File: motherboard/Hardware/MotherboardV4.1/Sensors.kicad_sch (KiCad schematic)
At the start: 33 parts, among them J401 0, J5 0, J6 0, J7 0

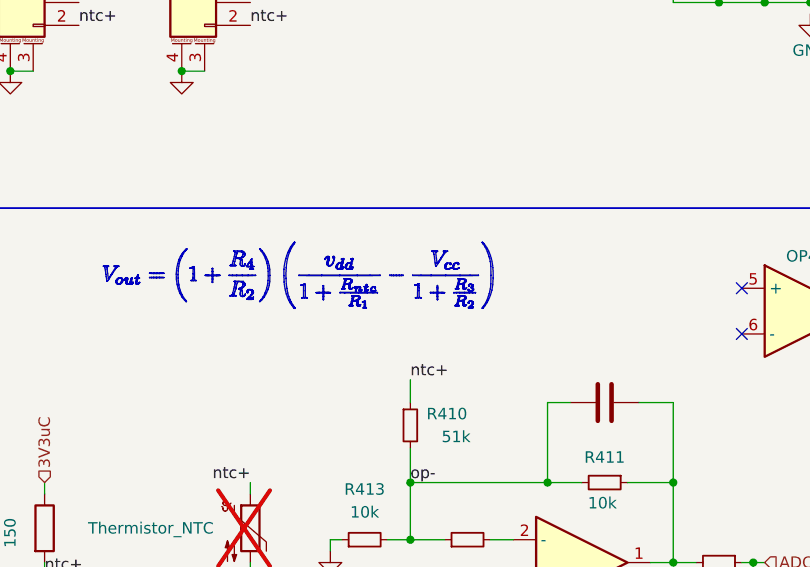
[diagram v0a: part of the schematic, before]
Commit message: working on thermal
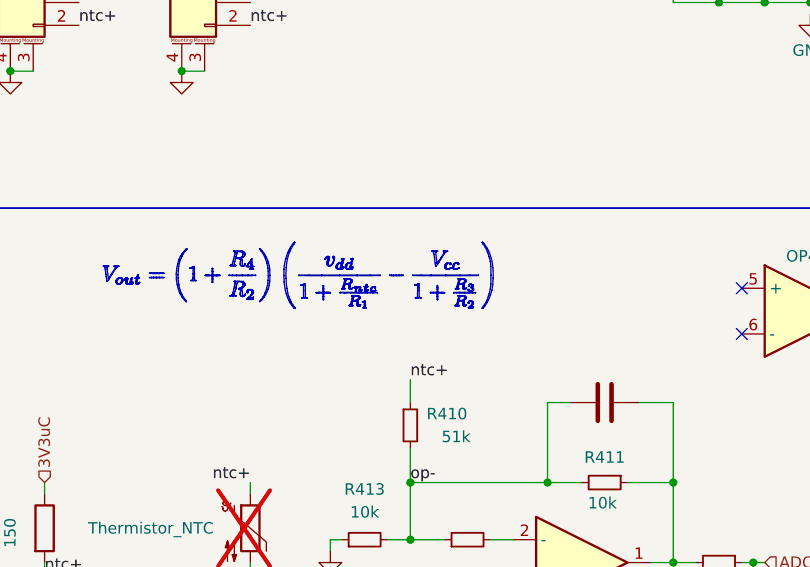
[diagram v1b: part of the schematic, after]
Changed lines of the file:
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@@
 	)
 	(arc
-		(start 90.1269 103.4387)
-		(mid 90.1288 103.4331)
-		(end 90.1339 103.4304)
+		(start 90.1339 103.4304)
+		(mid 90.134 103.4496)
+		(end 90.1269 103.4387)
 		(stroke
 			(width 0.08)
@@
 	)
 	(arc
-		(start 104.2505 108.8744)
-		(mid 104.2414 108.8715)
-		(end 104.24 108.8626)
+		(start 104.24 108.8626)
+		(mid 104.2608 108.8638)
+		(end 104.2505 108.8744)
 		(stroke
 			(width 0.08)
@@
 	)
 	(arc
-		(start 93.9377 106.897)
-		(mid 93.9501 106.9015)
-		(end 93.9446 106.9117)
+		(start 93.9446 106.9117)
+		(mid 93.9291 106.9062)
+		(end 93.9377 106.897)
 		(stroke
 			(width 0.08)
@@
 	)
 	(arc
-		(start 91.2932 107.5106)
-		(mid 91.2925 107.5121)
-		(end 91.2929 107.5181)
+		(start 91.2929 107.5181)
+		(mid 91.2904 107.5149)
+		(end 91.2932 107.5106)
 		(stroke
 			(width 0.08)
@@
 	)
 	(arc
-		(start 103.17 106.7418)
-		(mid 103.1741 106.7445)
-		(end 103.171 106.7481)
+		(start 103.171 106.7481)
+		(mid 103.1705 106.7481)
+		(end 103.17 106.7418)
 		(stroke
 			(width 0.08)

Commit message: worked on thermals
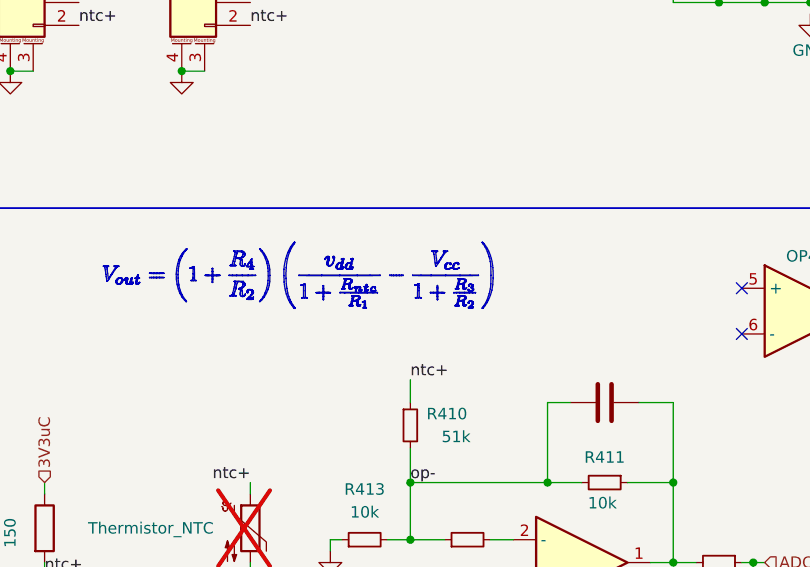
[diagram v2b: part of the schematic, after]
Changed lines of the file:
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@@
 	)
 	(arc
-		(start 90.1339 103.4304)
-		(mid 90.134 103.4496)
-		(end 90.1269 103.4387)
+		(start 90.1269 103.4387)
+		(mid 90.1288 103.4331)
+		(end 90.1339 103.4304)
 		(stroke
 			(width 0.08)
@@
 	)
 	(arc
-		(start 104.24 108.8626)
-		(mid 104.2608 108.8638)
-		(end 104.2505 108.8744)
+		(start 104.2505 108.8744)
+		(mid 104.2414 108.8715)
+		(end 104.24 108.8626)
 		(stroke
 			(width 0.08)
@@
 	)
 	(arc
-		(start 93.9446 106.9117)
-		(mid 93.9291 106.9062)
-		(end 93.9377 106.897)
+		(start 93.9377 106.897)
+		(mid 93.9501 106.9015)
+		(end 93.9446 106.9117)
 		(stroke
 			(width 0.08)
@@
 	)
 	(arc
-		(start 91.2929 107.5181)
-		(mid 91.2904 107.5149)
-		(end 91.2932 107.5106)
+		(start 91.2932 107.5106)
+		(mid 91.2925 107.5121)
+		(end 91.2929 107.5181)
 		(stroke
 			(width 0.08)
@@
 	)
 	(arc
-		(start 103.171 106.7481)
-		(mid 103.1705 106.7481)
-		(end 103.17 106.7418)
+		(start 103.17 106.7418)
+		(mid 103.1741 106.7445)
+		(end 103.171 106.7481)
 		(stroke
 			(width 0.08)
